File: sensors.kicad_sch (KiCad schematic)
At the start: 6 parts, among them U3 BMP390, U4 LSM6DSO32TR

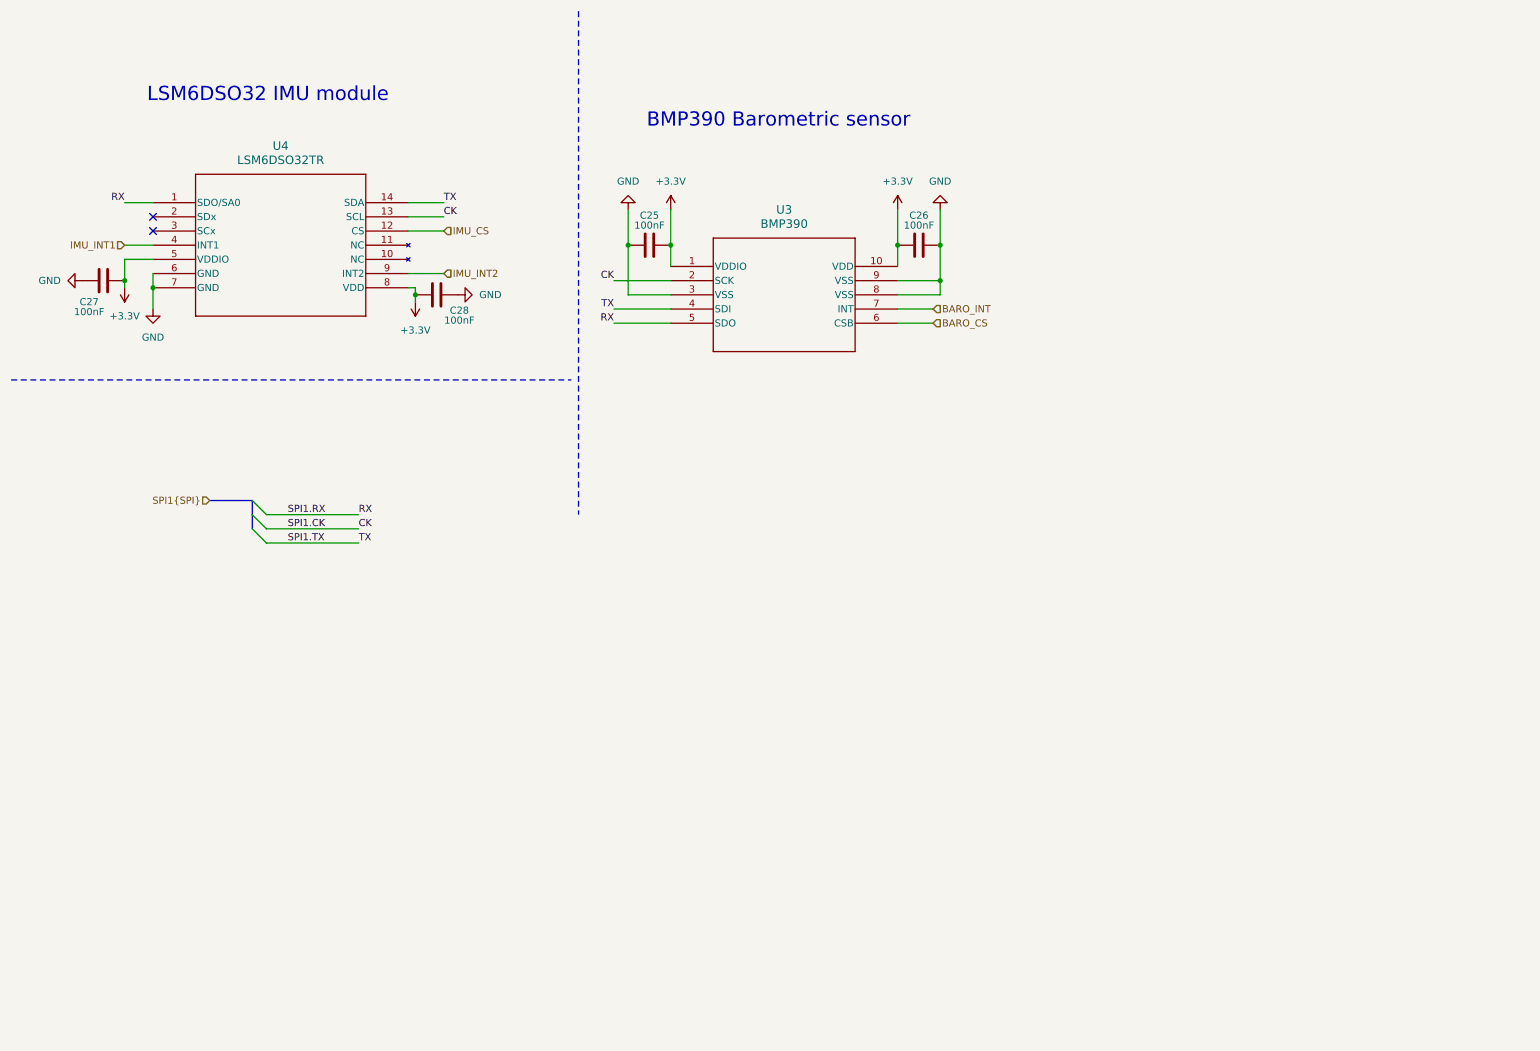
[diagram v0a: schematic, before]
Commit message: bozza layout pcb
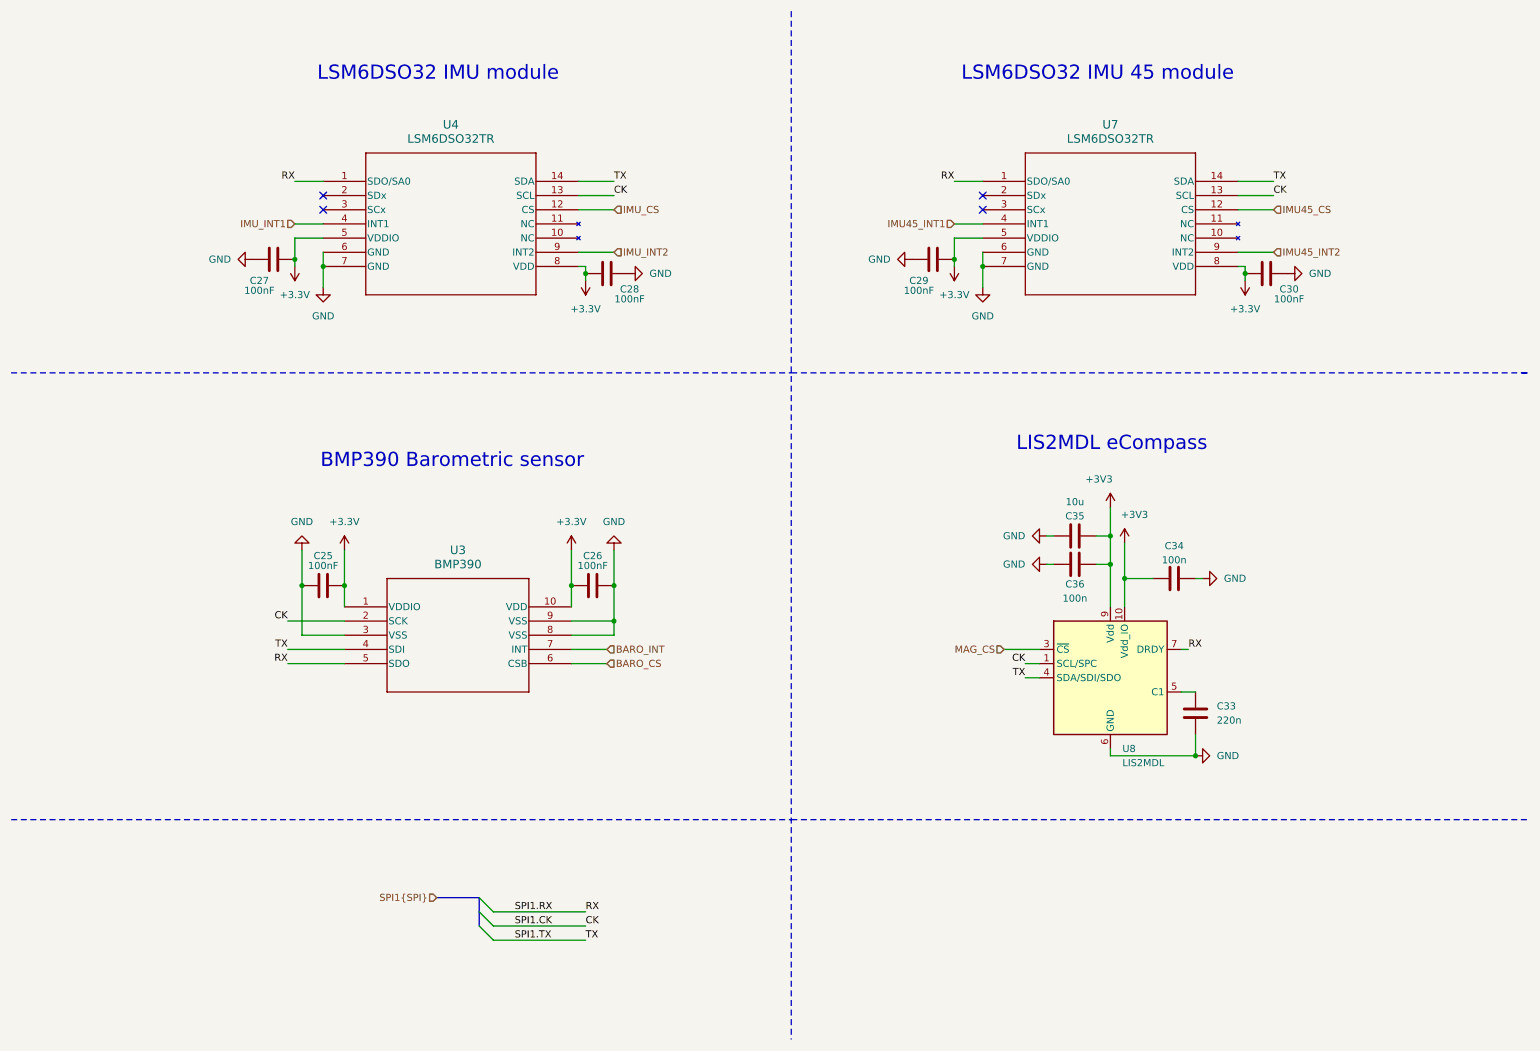
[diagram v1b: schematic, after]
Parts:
- added C29, C30: 100nF, Capacitor_SMD:C_0603_1608Metric_Pad1.08x0.95mm_HandSolder, symbol Device:C
- added C33: 220n, Capacitor_SMD:C_0603_1608Metric_Pad1.08x0.95mm_HandSolder, symbol Device:C
- added C34, C36: 100n, Capacitor_SMD:C_0603_1608Metric_Pad1.08x0.95mm_HandSolder, symbol Device:C
- added C35: 10u, Capacitor_SMD:C_0603_1608Metric_Pad1.08x0.95mm_HandSolder, symbol Device:C
- added U7: LSM6DSO32TR, LSM6DSO32TR:LGA-14L_2P5X3X0P83_STM-M, symbol 2024-10-18_09-38-35:LSM6DSO32TR
- added U8: LIS2MDL, Package_LGA:LGA-12_2x2mm_P0.5mm, symbol Sensor_Magnetic:LIS2MDL
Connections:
- net +3.3V: now also C29.2, C30.2, U7.5 (VDDIO), U7.8 (VDD)
- net CK: now also U7.13 (SCL), U8.1 (SCL/SPC)
- net GND: now also C29.1, C30.1, C33.2, C34.2, C35.2, C36.1, U7.6 (GND), U7.7 (GND), U8.6 (GND), U8.8 (GND)
- net RX: now also U7.1 (SDO/SA0), U8.7 (DRDY)
- net SPI1.TX: now also U7.14 (SDA), U8.4 (SDA/SDI/SDO)
- new net: C33.1, U8.5 (C1)
- new net +3V3: C34.1, C35.1, C36.2, U8.10 (Vdd_IO), U8.9 (Vdd)
- new net IMU45_CS: U7.12 (CS)
- new net IMU45_INT1: U7.4 (INT1)
- new net IMU45_INT2: U7.9 (INT2)
- new net MAG_CS: U8.3 (~{CS})
- no-connect marks 2 -> 4
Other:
- note added: "LIS2MDL eCompass"
- note added: "LSM6DSO32 IMU 45 module"
- moved on the sheet: C25, C26, C27, C28, U3, U4
